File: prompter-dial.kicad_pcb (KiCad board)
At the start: 2 copper layers, 75 x 100 mm, 8 parts, among them J1 PROMPTER WHEEL, SW1 JUMP_B, SW2 RUN, U1 ATtiny85-20S

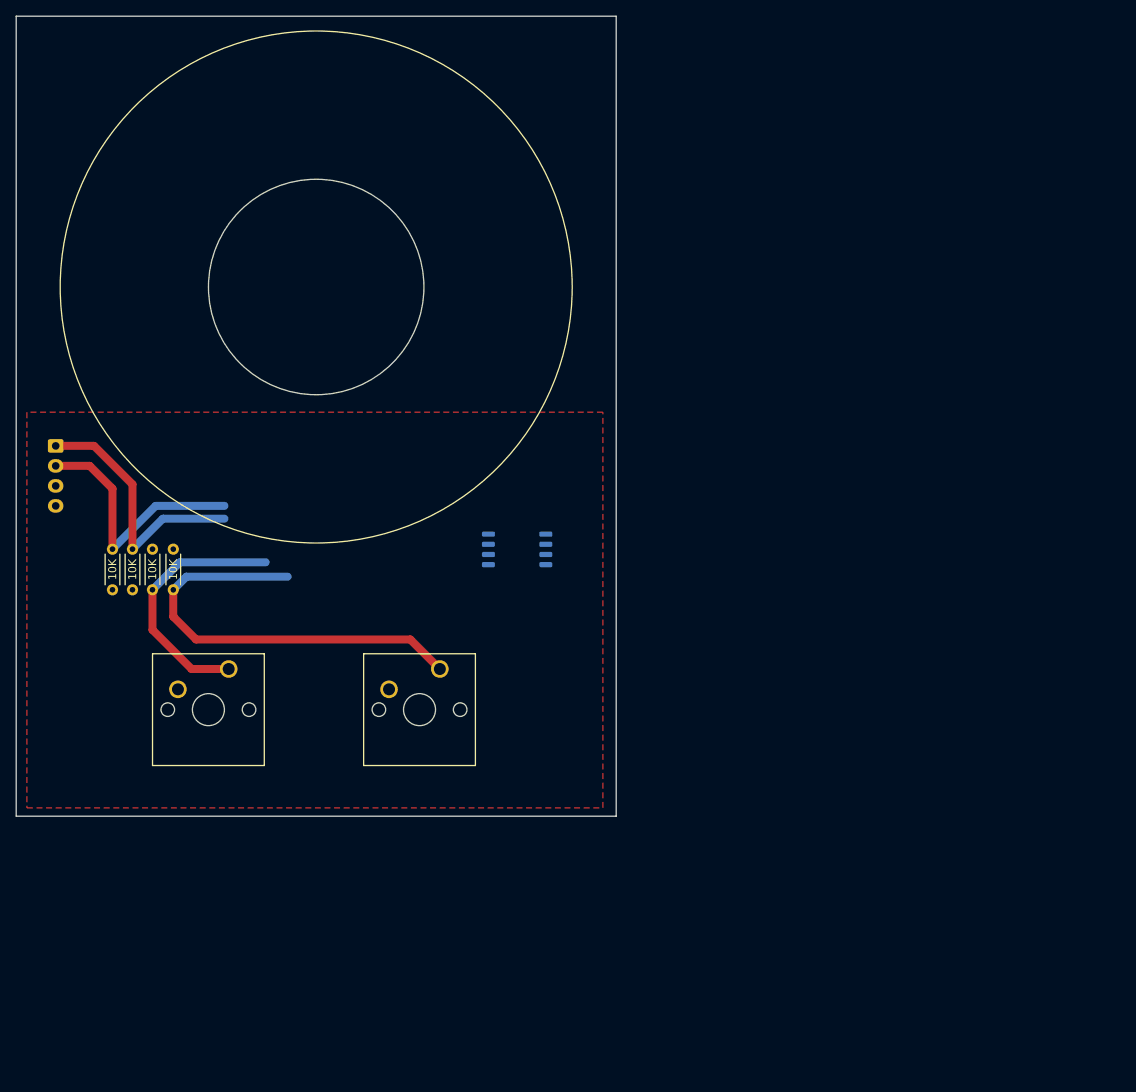
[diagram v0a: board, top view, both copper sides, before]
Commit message: Update prompter-dial.kicad_pcb
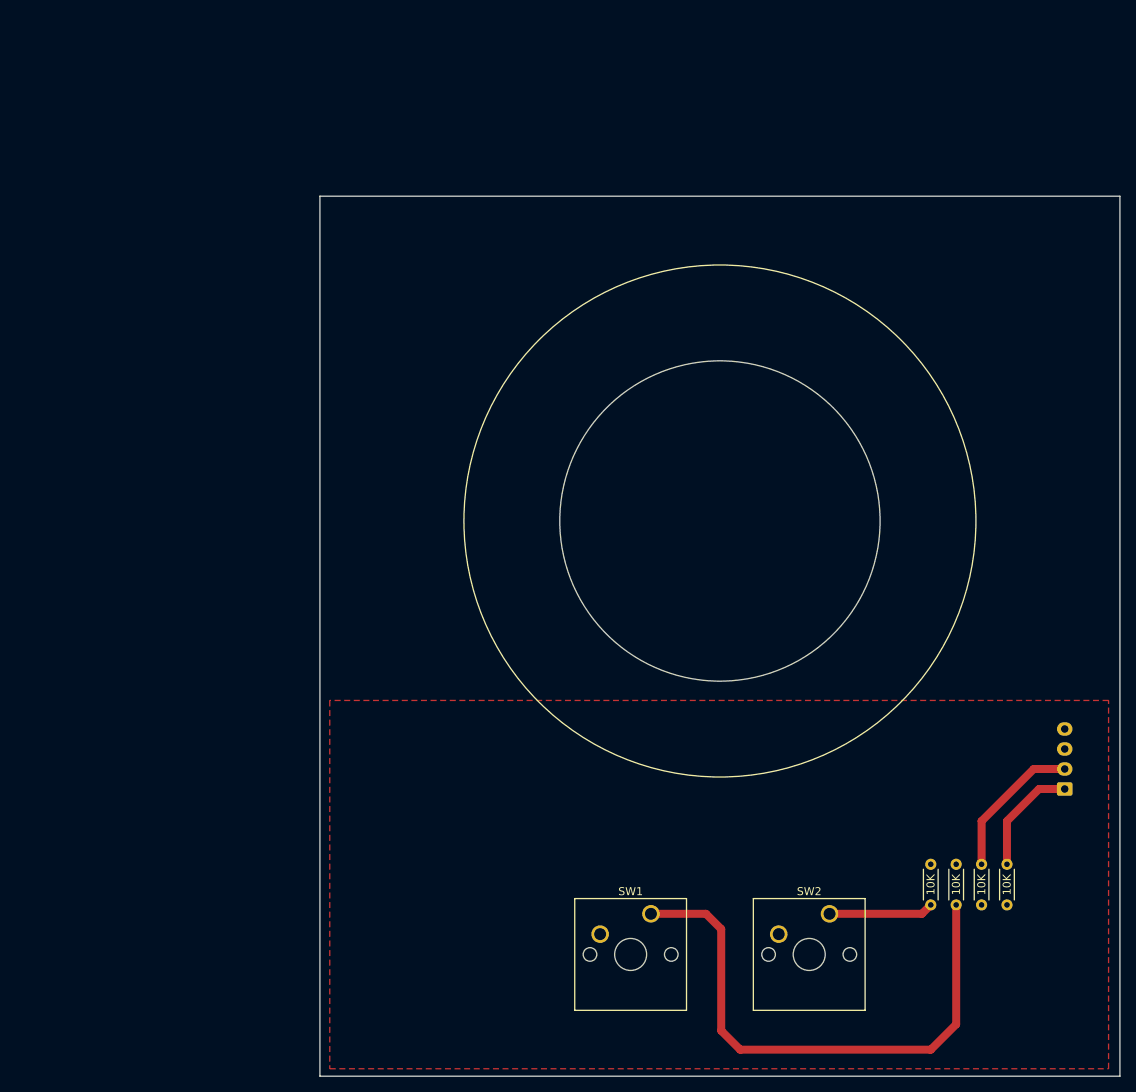
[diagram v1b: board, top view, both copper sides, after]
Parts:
- removed U1: ATtiny85-20S, Package_SO:SOIC-8_5.3x5.3mm_P1.27mm
- SW1: value JUMP_B -> JUMP
- moved J1 133.2 mm to (162.0, 115.0), turned to 90 degrees
- moved R6 116.2 mm to (154.8, 129.5)
- moved R5 115.6 mm to (151.6, 129.5)
- moved R1 107.9 mm to (148.4, 129.5)
- moved R2 102.6 mm to (145.3, 129.5)
- moved SW1 61.0 mm to (110.3, 130.7)
- moved SW2 57.5 mm to (132.6, 130.7)
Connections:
- net JUMP_B renamed JUMP
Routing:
- net RUN: track 54.4 -> 13.1 mm
- net JUMP: track 32.1 -> 68.9 mm
- net ENC_A: track 32.8 -> 14.3 mm
- net ENC_B: track 32.1 -> 18.5 mm
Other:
- board size 75 x 100 mm -> 100 x 110 mm
